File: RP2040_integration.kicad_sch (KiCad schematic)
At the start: 33 parts, among them J1 USB_B_Micro, J2 Conn_01x02, U1 NCP1117-3.3_SOT223, U2 W25Q128JVS, U3 RP2040, Y1 ABM8-272-T3

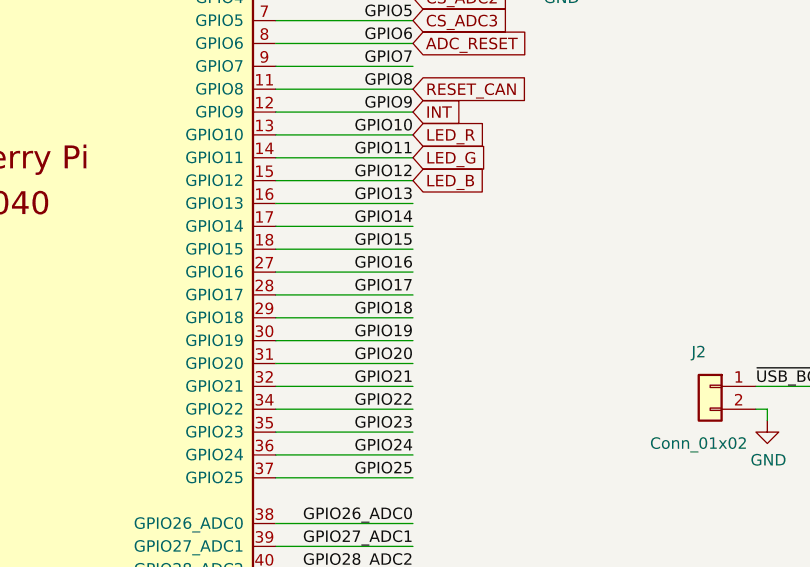
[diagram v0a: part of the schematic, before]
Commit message: Schematic ok (je crois)
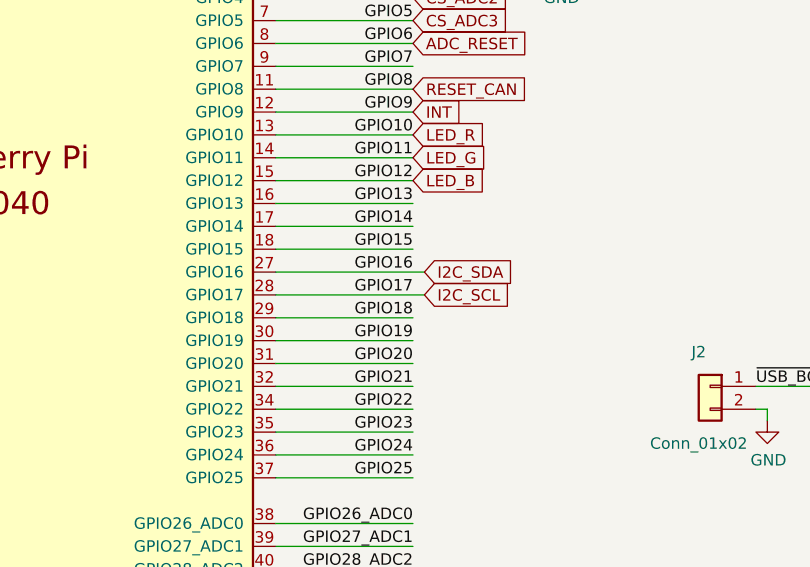
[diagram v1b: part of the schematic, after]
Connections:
- net GPIO16 renamed I2C_SDA
- net GPIO17 renamed I2C_SCL
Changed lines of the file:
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@@
 	(wire
 		(pts
-			(xy 132.08 162.56) (xy 147.32 162.56)
+			(xy 132.08 162.56) (xy 148.59 162.56)
 		)
 		(stroke
@@
 	(wire
 		(pts
-			(xy 132.08 160.02) (xy 147.32 160.02)
+			(xy 132.08 160.02) (xy 148.59 160.02)
 		)
 		(stroke
@@
 		)
 	)
+	(global_label "I2C_SCL"
+		(shape input)
+		(at 148.59 162.56 0)
+		(fields_autoplaced yes)
+		(effects
+			(font
+				(size 1.27 1.27)
+			)
+			(justify left)
+		)
+		(property "Intersheetrefs" "${INTERSHEET_REFS}"
+			(at 159.1347 162.56 0)
+			(effects
+				(font
+					(size 1.27 1.27)
+				)
+				(justify left)
+				(hide yes)
+			)
+		)
+	)
 	(global_label "INT"
 		(shape input)
@@
 			(effects
 				(font
+					(size 1.27 1.27)
+				)
+				(justify left)
+				(hide yes)
+			)
+		)
+	)
+	(global_label "I2C_SDA"
+		(shape input)
+		(at 148.59 160.02 0)
+		(fields_autoplaced yes)
+		(effects
+			(font
+				(size 1.27 1.27)
+			)
+			(justify left)
+		)
+		(property "Intersheetrefs" "${INTERSHEET_REFS}"
+			(at 159.1952 160.02 0)
+			(effects
+				(font

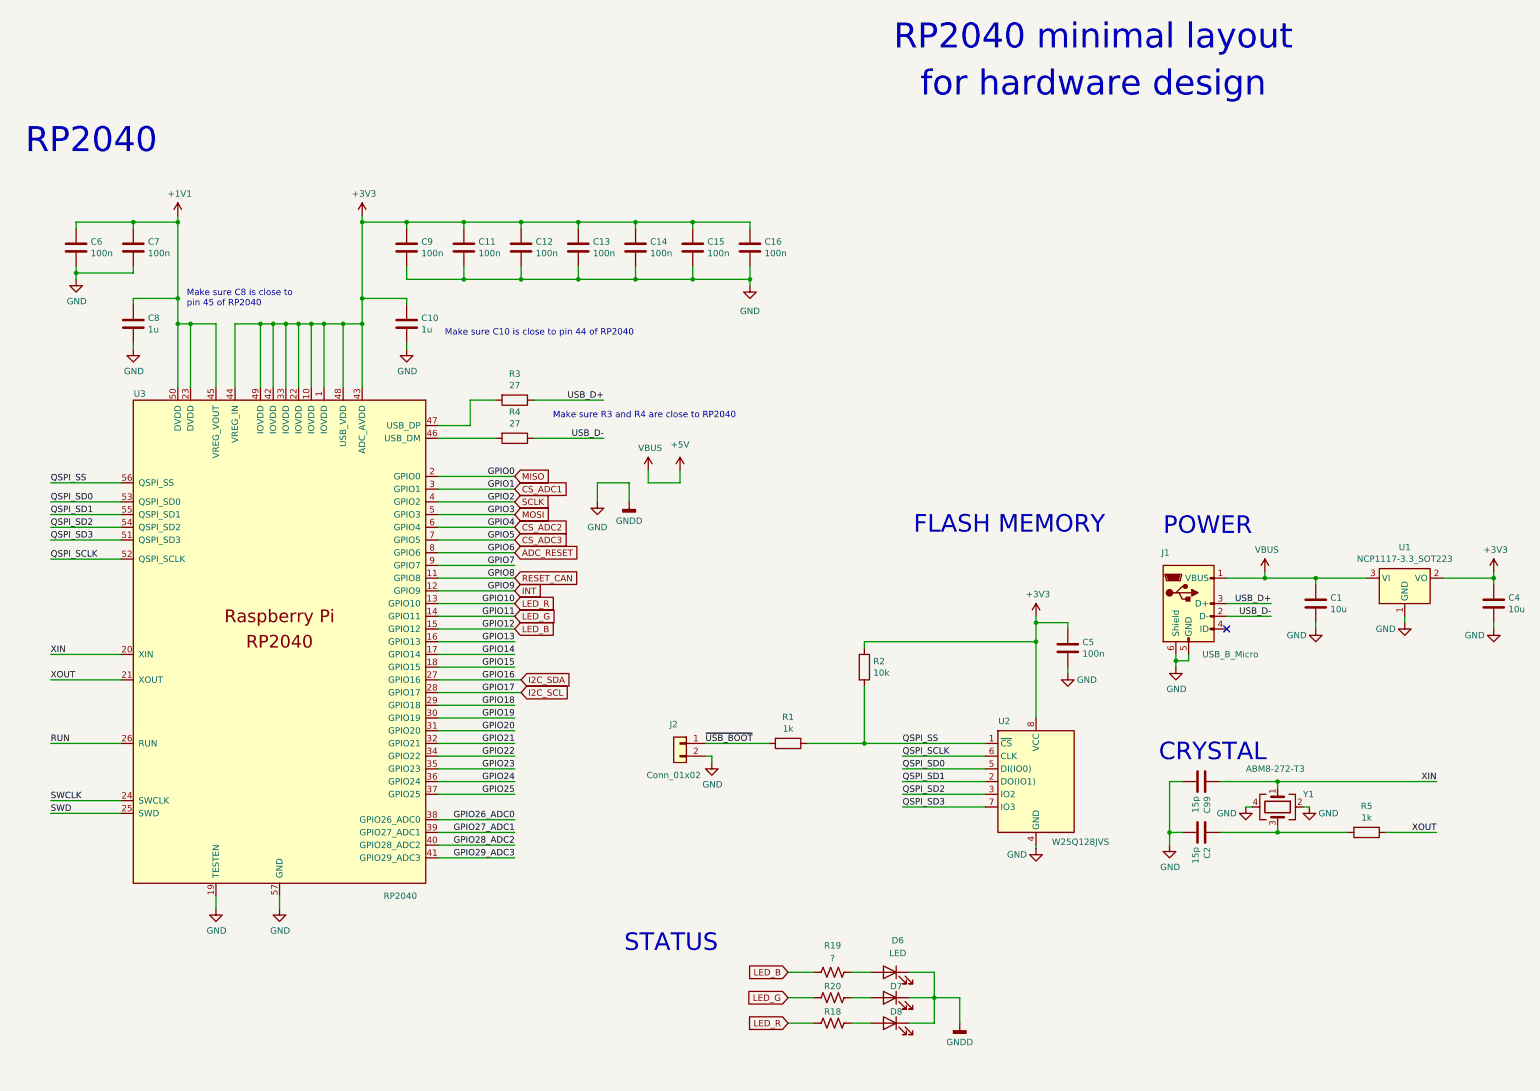
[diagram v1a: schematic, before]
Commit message: Last Push pour que tu check, après je commence le Layout
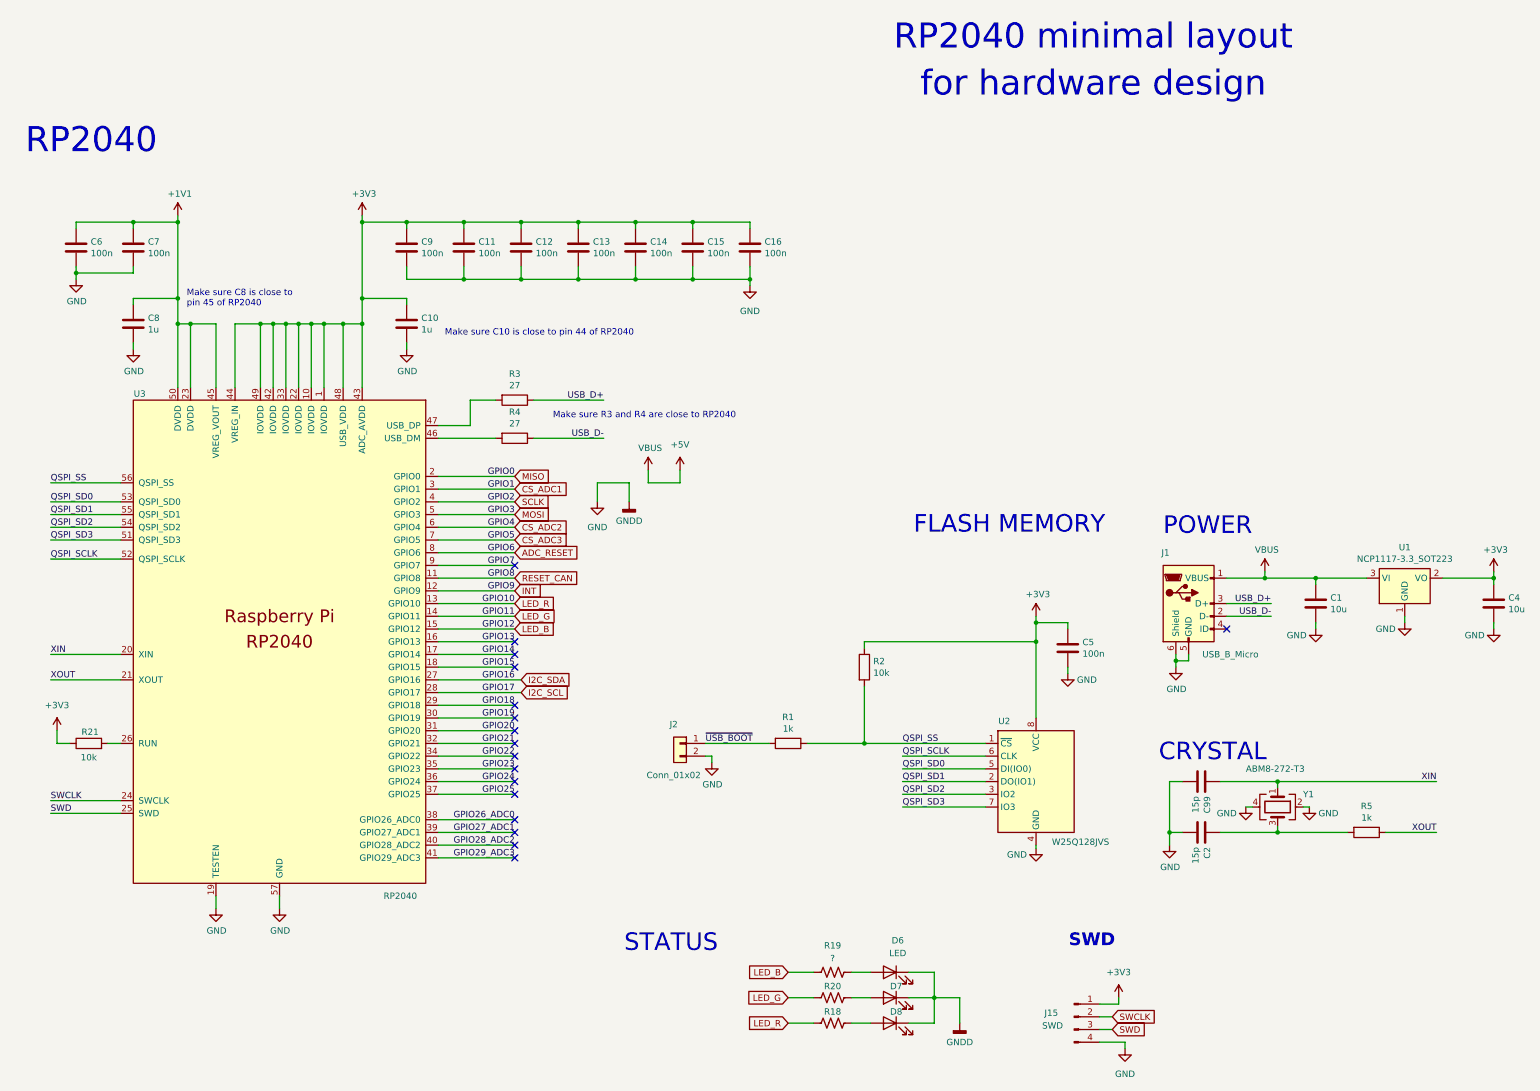
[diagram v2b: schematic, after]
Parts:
- added J15: SWD, Connector_PinHeader_2.54mm:PinHeader_1x04_P2.54mm_Vertical, symbol Connector:Conn_01x04_Pin
- added R21: 10k, Resistor_SMD:R_0603_1608Metric, symbol DPR_devices:R
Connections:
- net +3V3: now also J15.1 (Pin_1), R21.1
- net GND: now also J15.4 (Pin_4)
- net SWCLK: now also J15.2 (Pin_2)
- net SWD: now also J15.3 (Pin_3)
- net RUN: no longer names the net of U3.26 (RUN)
- net RUN: now also R21.2
- no-connect marks 1 -> 17
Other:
- note added: "SWD"

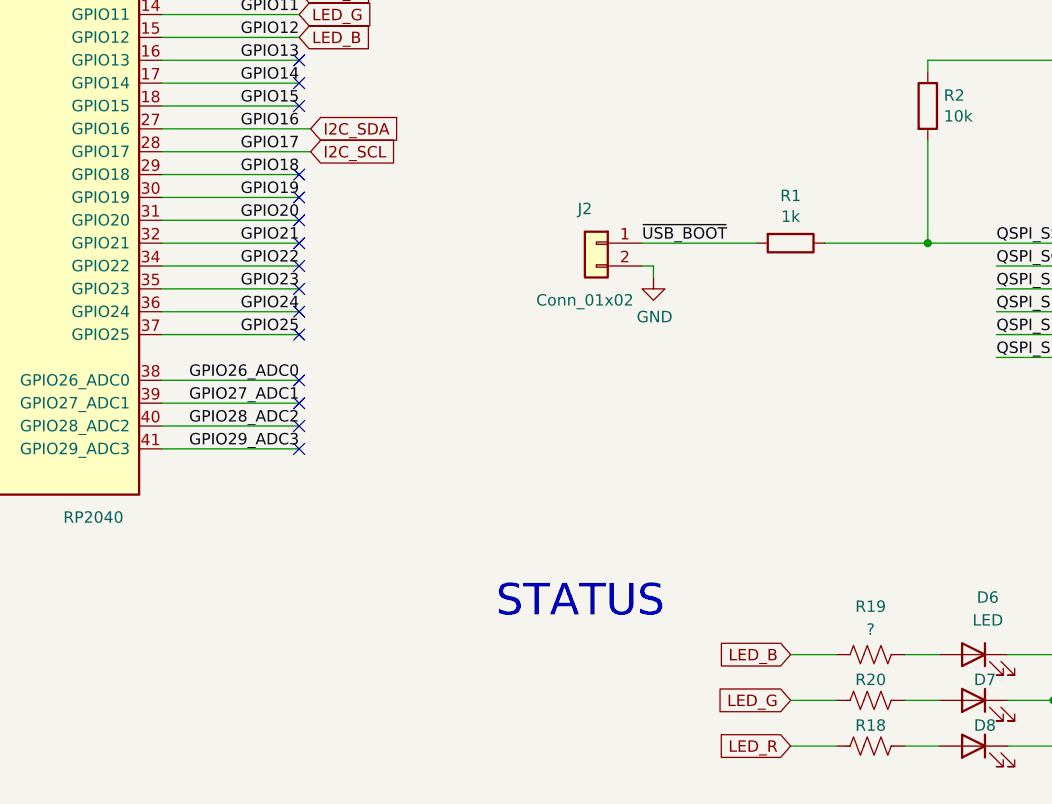
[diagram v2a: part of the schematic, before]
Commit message: Finito je te laisse check
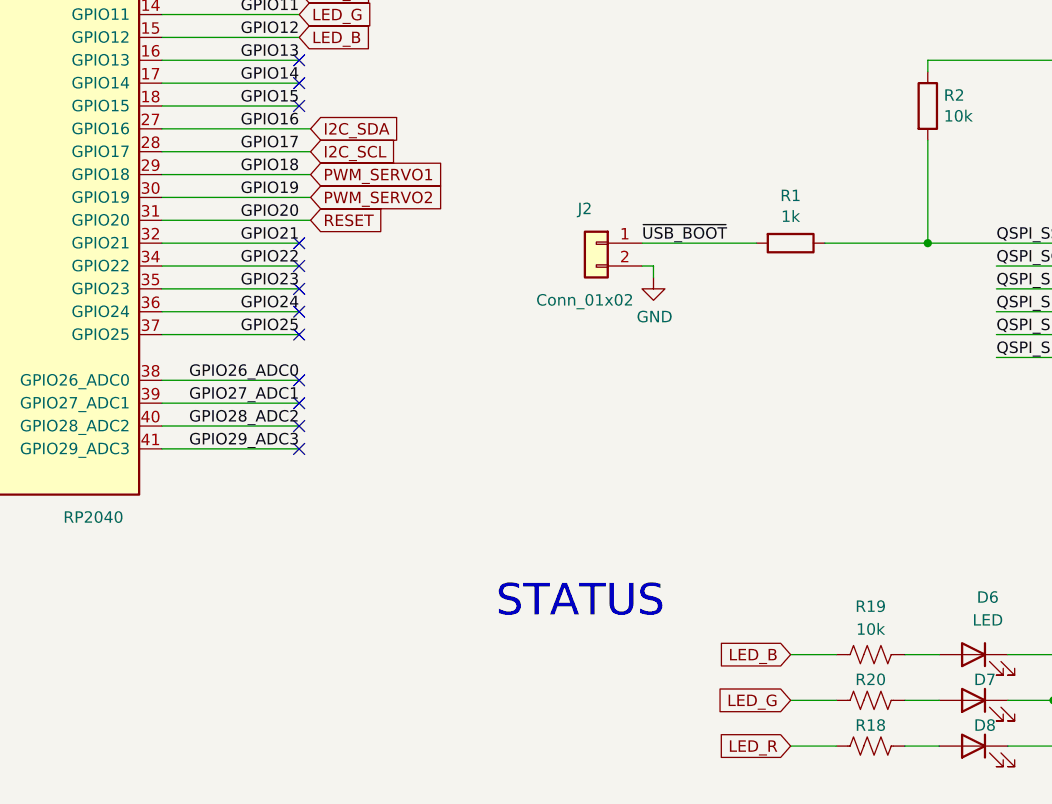
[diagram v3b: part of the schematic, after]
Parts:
- R18, R20: value R_US -> 10k
- R19: value ? -> 10k
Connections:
- net GPIO18 renamed PWM_SERVO1
- net GPIO19 renamed PWM_SERVO2
- net GPIO20 renamed RESET
- no-connect marks 17 -> 14
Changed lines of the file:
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@@
 	)
 	(no_connect
-		(at 147.32 170.18)
-	)
-	(no_connect
 		(at 147.32 157.48)
 	)
@@
 	)
 	(no_connect
-		(at 147.32 165.1)
-	)
-	(no_connect
 		(at 147.32 137.16)
 	)
@@
 	)
 	(no_connect
-		(at 147.32 167.64)
-	)
-	(no_connect
 		(at 147.32 190.5)
 	)
@@
 	(wire
 		(pts
-			(xy 132.08 167.64) (xy 147.32 167.64)
+			(xy 132.08 167.64) (xy 148.59 167.64)
 		)
 		(stroke
@@
 	(wire
 		(pts
-			(xy 132.08 165.1) (xy 147.32 165.1)
+			(xy 132.08 165.1) (xy 148.59 165.1)
 		)
 		(stroke
@@
 	(wire
 		(pts
-			(xy 132.08 170.18) (xy 147.32 170.18)
+			(xy 132.08 170.18) (xy 148.59 170.18)
 		)
 		(stroke
@@
 		)
 	)
+	(global_label "PWM_SERVO1"
+		(shape input)
+		(at 148.59 165.1 0)
+		(fields_autoplaced yes)
+		(effects
+			(font
+				(size 1.27 1.27)
+			)
+			(justify left)
+		)
+		(property "Intersheetrefs" "${INTERSHEET_REFS}"
+			(at 163.9727 165.1 0)
+			(effects
+				(font
+					(size 1.27 1.27)
+				)
+				(justify left)
+				(hide yes)
+			)
+		)
+	)
 	(global_label "ADC_RESET"
 		(shape input)
@@
 		)
 	)
+	(global_label "RESET"
+		(shape input)
+		(at 148.59 170.18 0)
+		(fields_autoplaced yes)
+		(effects
+			(font
+				(size 1.27 1.27)
+			)
+			(justify left)
+		)
+		(property "Intersheetrefs" "${INTERSHEET_REFS}"
+			(at 157.3203 170.18 0)
+			(effects
+				(font
+					(size 1.27 1.27)
+				)
+				(justify left)
+				(hide yes)
+			)
+		)
+	)
 	(global_label "I2C_SCL"
 		(shape input)
@@
 		)
 	)
+	(global_label "PWM_SERVO2"
+		(shape input)
+		(at 148.59 167.64 0)
+		(fields_autoplaced yes)
+		(effects
+			(font
+				(size 1.27 1.27)
+			)
+			(justify left)
+		)
+		(property "Intersheetrefs" "${INTERSHEET_REFS}"
+			(at 163.9727 167.64 0)
+			(effects
+				(font
+					(size 1.27 1.27)
+				)
+				(justify left)
+				(hide yes)
+			)
+		)
+	)
 	(global_label "LED_B"
 		(shape input)
@@
 			)
 			(stroke
-				(width 0.254)
+				(width 0.7)
 				(type solid)
-				(color 0 0 132 1)
+				(color 0 0 255 1)
 			)
 			(fill
@@
 			)
 		)
-		(property "Description" ""
+		(property "Description" "USB Micro Type B connector"
 			(at 281.94 144.78 0)
 			(effects
@@
 					(size 1.27 1.27)
 				)
+				(hide yes)
 			)
 		)
@@
 			)
 		)
-		(property "Value" "R_US"
+		(property "Value" "10k"
 			(at 210.82 224.79 90)
 			(effects
@@
 			)
 		)
-		(property "Value" "?"
+		(property "Value" "10k"
 			(at 210.82 215.646 90)
 			(effects
@@
 			)
 		)
-		(property "Value" "R_US"
+		(property "Value" "10k"
 			(at 210.82 219.71 90)
 			(effects
